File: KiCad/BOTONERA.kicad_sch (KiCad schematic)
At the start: 16 parts, among them SW1 SW_Push, SW2 SW_Push, SW3 SW_Push, SW4 SW_Push, SW5 SW_Push, SW6 SW_Push, SW7 SW_Push, SW8 SW_Push

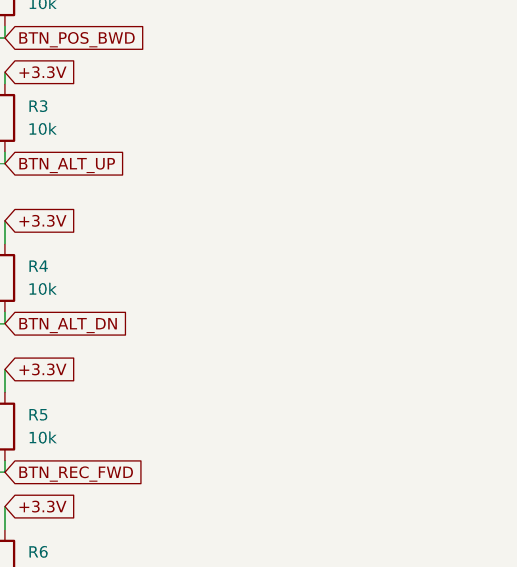
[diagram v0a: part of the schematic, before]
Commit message: Modificacio
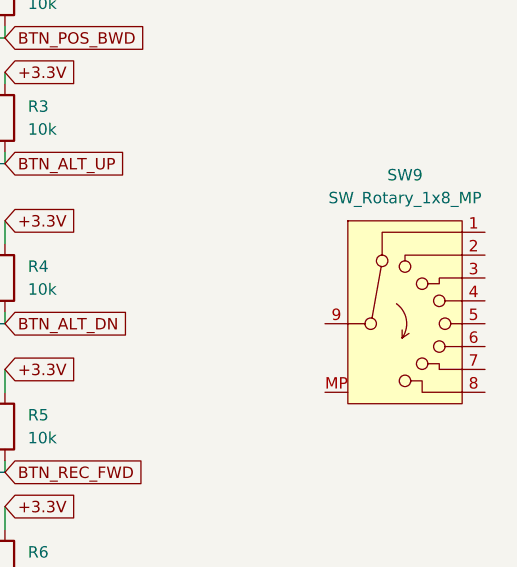
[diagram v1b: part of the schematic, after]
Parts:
- added SW9: SW_Rotary_1x8_MP, symbol Switch:SW_Rotary_1x8_MP
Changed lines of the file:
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@@
+	)
+	(symbol
+		(lib_id "Switch:SW_Rotary_1x8_MP")
+		(at 148.59 102.87 0)
+		(unit 1)
+		(exclude_from_sim no)
+		(in_bom yes)
+		(on_board yes)
+		(dnp no)
+		(fields_autoplaced yes)
+		(property "Reference" "SW9"
+			(at 147.32 86.36 0)
+			(effects
+				(font
+					(size 1.27 1.27)
+				)
+			)
+		)
+		(property "Value" "SW_Rotary_1x8_MP"
+			(at 147.32 88.9 0)
+			(effects
+				(font
+					(size 1.27 1.27)
+				)
+			)
+		)
+		(property "Footprint" ""
+			(at 147.32 102.87 0)
+			(effects
+				(font
+					(size 1.27 1.27)
+				)
+				(hide yes)
+			)
+		)
+		(property "Datasheet" "~"
+			(at 147.32 102.87 0)
+			(effects
+				(font
+					(size 1.27 1.27)
+				)
+				(hide yes)
+			)
+		)
+		(property "Description" "Rotary switch 1x8, SP8T with mount point"
+			(at 148.59 102.87 0)
+			(effects
+				(font
+					(size 1.27 1.27)
+				)
+				(hide yes)
+			)
+		)
+		(pin "9"
+		)
+		(pin "4"
+		)
+		(pin "1"
+		)
+		(pin "MP"
+		)
+		(pin "2"
+		)
+		(pin "3"
+		)
+		(pin "5"
+		)
+		(pin "6"
+		)
+		(pin "8"
+		)
+		(pin "7"
+		)
+		(instances
+			(project ""
+				(path "/b6401b4f-5426-49b8-bb2e-8ecdb19989ef/d2dca798-87db-444b-885e-260b410044df"
+					(reference "SW9")
+					(unit 1)
+				)
+			)
+		)
 	)
 	(symbol

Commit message: Millora
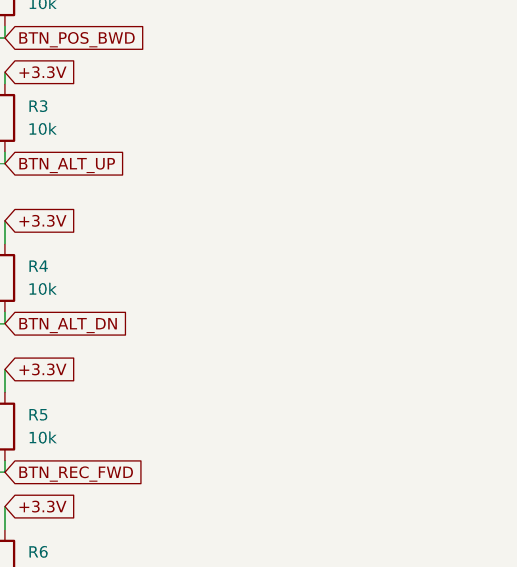
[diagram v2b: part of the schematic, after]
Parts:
- removed SW9: SW_Rotary_1x8_MP, symbol Switch:SW_Rotary_1x8_MP
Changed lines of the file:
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@@
-	)
-	(symbol
-		(lib_id "Switch:SW_Rotary_1x8_MP")
-		(at 148.59 102.87 0)
-		(unit 1)
-		(exclude_from_sim no)
-		(in_bom yes)
-		(on_board yes)
-		(dnp no)
-		(fields_autoplaced yes)
-		(property "Reference" "SW9"
-			(at 147.32 86.36 0)
-			(effects
-				(font
-					(size 1.27 1.27)
-				)
-			)
-		)
-		(property "Value" "SW_Rotary_1x8_MP"
-			(at 147.32 88.9 0)
-			(effects
-				(font
-					(size 1.27 1.27)
-				)
-			)
-		)
-		(property "Footprint" ""
-			(at 147.32 102.87 0)
-			(effects
-				(font
-					(size 1.27 1.27)
-				)
-				(hide yes)
-			)
-		)
-		(property "Datasheet" "~"
-			(at 147.32 102.87 0)
-			(effects
-				(font
-					(size 1.27 1.27)
-				)
-				(hide yes)
-			)
-		)
-		(property "Description" "Rotary switch 1x8, SP8T with mount point"
-			(at 148.59 102.87 0)
-			(effects
-				(font
-					(size 1.27 1.27)
-				)
-				(hide yes)
-			)
-		)
-		(pin "9"
-		)
-		(pin "4"
-		)
-		(pin "1"
-		)
-		(pin "MP"
-		)
-		(pin "2"
-		)
-		(pin "3"
-		)
-		(pin "5"
-		)
-		(pin "6"
-		)
-		(pin "8"
-		)
-		(pin "7"
-		)
-		(instances
-			(project ""
-				(path "/b6401b4f-5426-49b8-bb2e-8ecdb19989ef/d2dca798-87db-444b-885e-260b410044df"
-					(reference "SW9")
-					(unit 1)
-				)
-			)
-		)
 	)
 	(symbol
